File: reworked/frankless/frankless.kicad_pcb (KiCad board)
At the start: 4 copper layers, 32 x 74 mm, 117 parts, among them J1 GPIO, J10 BAT 3V, J2 DEBUG, J3 1040310811, J4 SS-52100-004, J5 USB4215-03-A, J6 HC-HDMI0019T-1A, J7 PJ-320D, J8 UART, U1 TS3USB221RSER, U10 DS3231MZ+TRL, U11 CH334R, U2 USBLC6-2SC6, U3 AMS1117-3.3, U5 APS6404L-3SQR-SN, U6 W25Q128JVS, U7 RP2350, U8 TDA1387T, U9 LM358, Y1 ASE-12MHz, Y2 12Mhz, Y3 ASE-12MHz

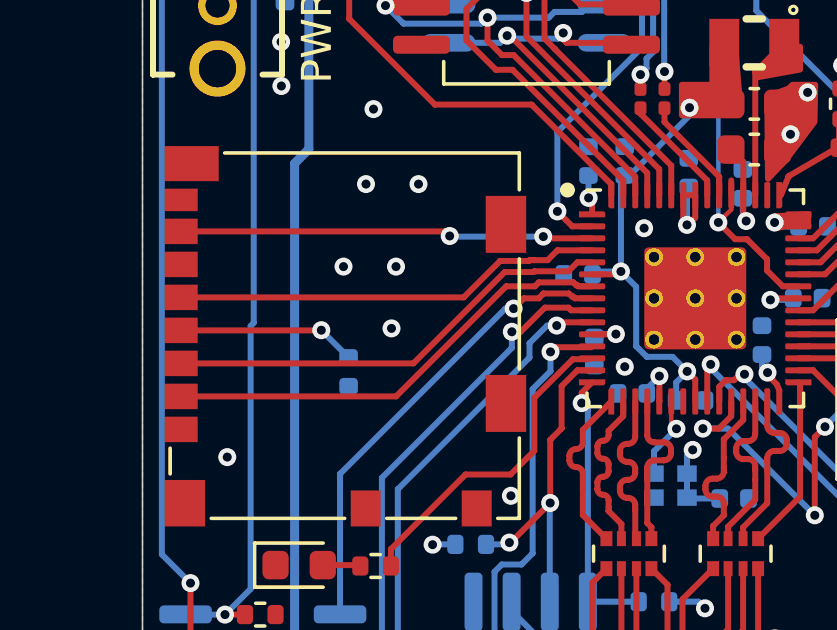
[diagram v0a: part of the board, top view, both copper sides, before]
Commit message: Patch a few minor issues.
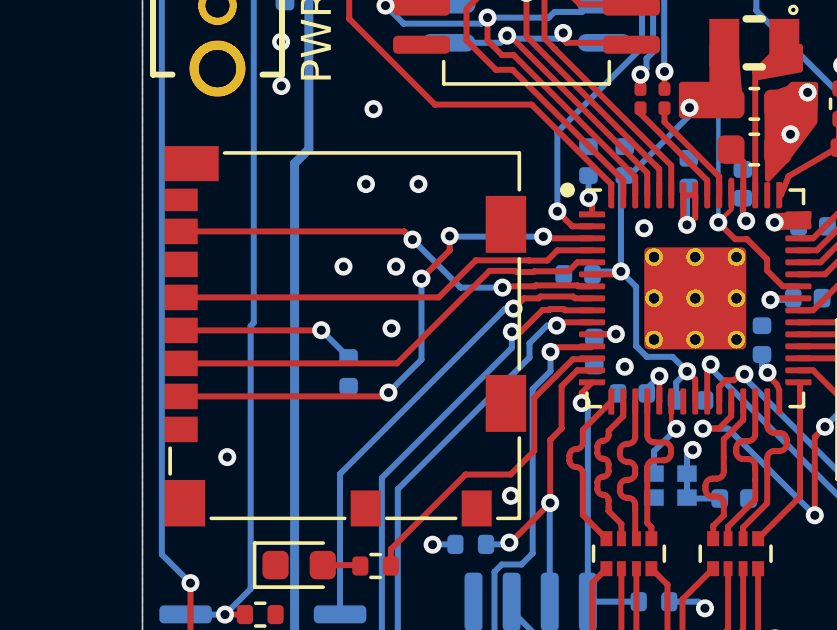
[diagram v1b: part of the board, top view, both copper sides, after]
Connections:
- net /RP2350A/GPI027/ADC1 renamed /RP2350A/GPIO27/ADC1
- C39 pad 2: +3V3 -> Net-(U11-VDD33_{LDO})
- C40 pad 2: +3V3 -> Net-(U11-VDD33_{LDO})
- U11 pad 13: +3V3 -> Net-(U11-VDD33_{LDO})
- U7 pad 3: /Micro SD/DAT0 -> /Micro SD/CDDAT3
- U7 pad 7: /Micro SD/CDDAT3 -> /Micro SD/DAT0
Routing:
- net Net-(U11-VDD33_{LDO}): track 0.00 -> 3.46 mm, vias 0 -> 1
- net +3V3: track 69.3 -> 65.8 mm, vias 25 -> 24
- net /Micro SD/CDDAT3: track 15.3 -> 18.0 mm, vias 0 -> 4
- net /Micro SD/DAT0: track 13.8 -> 14.5 mm
